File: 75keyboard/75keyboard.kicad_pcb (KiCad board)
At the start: 2 copper layers, 351 x 128 mm, 169 parts, among them SW1 SW_Push, SW10 SW_Push, SW11 SW_Push, SW12 SW_Push, SW13 SW_Push, SW14 SW_Push, SW15 SW_Push, SW16 SW_Push, SW17 SW_Push, SW18 SW_Push, SW19 SW_Push, SW2 SW_Push, SW20 SW_Push, SW21 SW_Push, SW22 SW_Push, SW23 SW_Push, SW24 SW_Push, SW25 SW_Push, SW26 SW_Push, SW27 SW_Push, SW28 SW_Push, SW29 SW_Push, SW3 SW_Push, SW30 SW_Push, SW31 SW_Push, SW32 SW_Push, SW33 SW_Push, SW34 SW_Push, SW35 SW_Push, SW36 SW_Push, SW37 SW_Push, SW38 SW_Push, SW39 SW_Push, SW4 SW_Push, SW40 SW_Push, SW41 SW_Push, SW42 SW_Push, SW43 SW_Push, SW44 SW_Push, SW45 SW_Push, SW46 SW_Push, SW47 SW_Push, SW48 SW_Push, SW49 SW_Push, SW5 SW_Push, SW50 SW_Push, SW51 SW_Push, SW52 SW_Push, SW53 SW_Push, SW54 SW_Push, SW55 SW_Push, SW56 SW_Push, SW57 SW_Push, SW58 SW_Push, SW59 SW_Push, SW6 SW_Push, SW60 SW_Push, SW61 SW_Push, SW62 SW_Push, SW63 SW_Push, SW64 SW_Push, SW65 SW_Push, SW66 SW_Push, SW67 SW_Push, SW68 SW_Push, SW69 SW_Push, SW7 SW_Push, SW70 SW_Push, SW71 SW_Push, SW72 SW_Push, SW73 SW_Push, SW74 SW_Push, SW75 SW_Push, SW76 SW_Push, SW77 SW_Push, SW78 SW_Push, SW79 SW_Push, SW8 SW_Push, SW80 SW_Push, SW81 SW_Push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

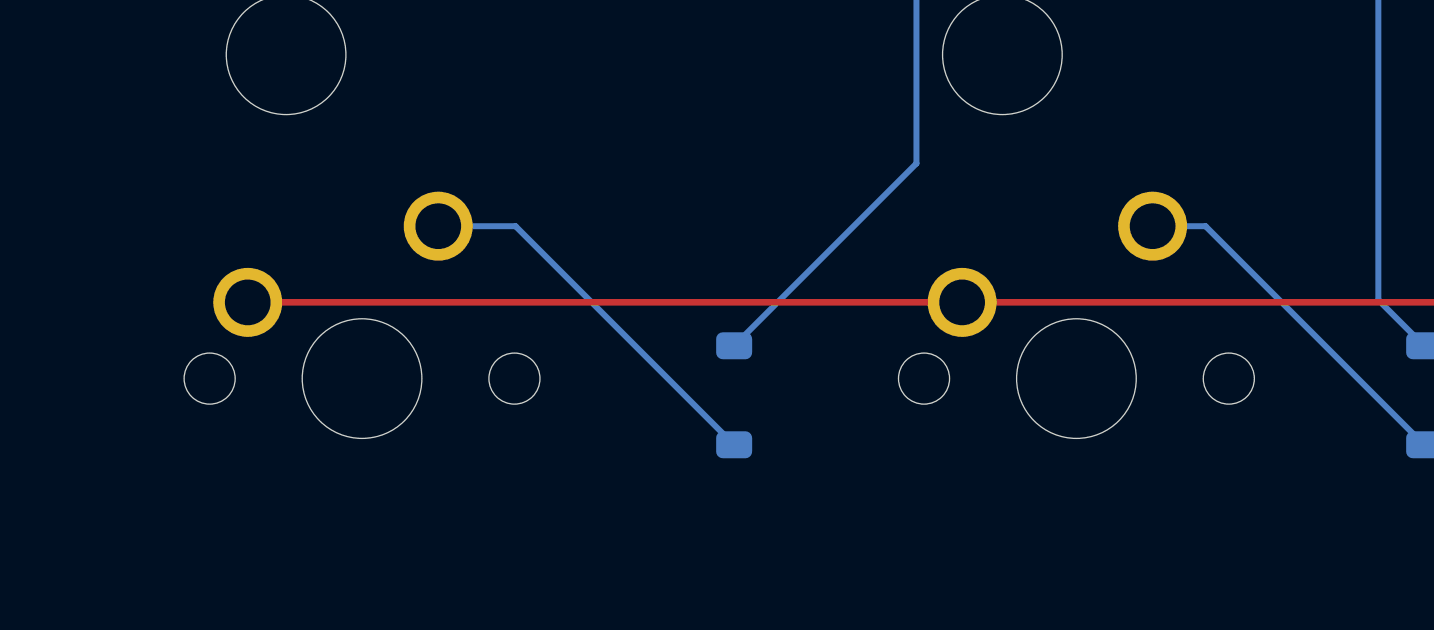
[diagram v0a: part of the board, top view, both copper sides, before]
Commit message: .
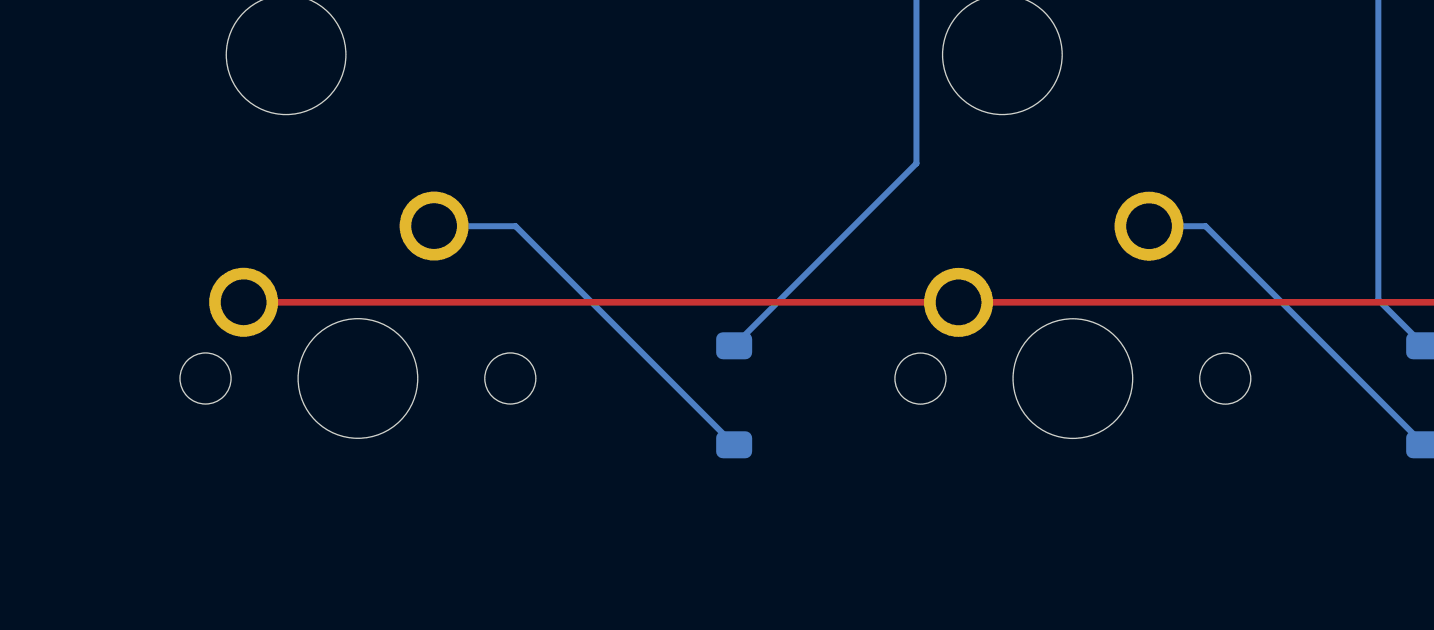
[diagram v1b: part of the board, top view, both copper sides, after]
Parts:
- moved SW75 0.14 mm to (34.7, 135.7)
- moved SW76 0.12 mm to (58.6, 135.7)
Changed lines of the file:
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@@
 		(allow_soldermask_bridges_in_footprints no)
 		(tenting front back)
-		(grid_origin 14.2875 14.2875)
+		(grid_origin 22.86 30.9562)
 		(pcbplotparams
 			(layerselection 0x00000000_00000000_55555555_5755f5ff)
@@
 	(footprint "MX_Solderable:MX-Solderable-1.25U"
 		(layer "F.Cu")
-		(at 34.885 135.7312)
+		(at 34.74745 135.7275)
 		(property "Reference" "SW75"
 			(at 0 3.175 0)
@@
 	(footprint "MX_Solderable:MX-Solderable-1.25U"
 		(layer "F.Cu")
-		(at 58.6975 135.7312)
+		(at 58.57875 135.7312)
 		(property "Reference" "SW76"
 			(at 0 3.175 0)
